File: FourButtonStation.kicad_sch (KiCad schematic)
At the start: 41 parts, among them J1 c8-inlet, J2 Conn_WallSocket, J3 I2C, J4 AVOX Adapter, J5 Conn_WallSocket, J6 USB_B_Micro, J7 Conn_WallSocket, J8 Conn_WallSocket, J9 I2C, K1 G5Q-1, K2 G5Q-1, K4 FINDER-36.11, K5 G5Q-1, Q1 MMBT3904, Q2 MMBT3904, Q3 MMBT3904, Q4 MMBT3904, Q5 MMBT3904, Q6 MMBT3904, SW3 RST, SW4 Boot, U1 CH340C, U2 radio-receiver, U3 ESP-07

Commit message: Schematic and routing
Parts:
- removed C1: TODO: 20u as SMD Package?, Capacitor_THT:CP_Radial_D5.0mm_P2.50mm, symbol Device:C_Polarized_Small
- removed D1: TODO: SMD Diodes Package, Diode_THT:D_DO-15_P2.54mm_Vertical_KathodeUp, symbol Device:D_Small
- removed D2, D3, D4: D_Small, Diode_THT:D_DO-15_P2.54mm_Vertical_KathodeUp, symbol Device:D_Small
- removed J2: Conn_WallSocket, TerminalBlock_Phoenix:TerminalBlock_Phoenix_MKDS-1,5-2_1x02_P5.00mm_Horizontal, symbol Connector:Conn_WallSocket
- removed J9: I2C, jlc_footprints:CONN-SMD_BM04B-SRSS-TB, symbol BM04B-SRSS-TB(LF)(SN):BM04B-SRSS-TB(LF)(SN)
- removed K1, K2, K5: G5Q-1, omron-g5sb-14:RELAY_G5SB-14_OMR, symbol Relay:G5Q-1
- removed K4: FINDER-36.11, omron-g5sb-14:RELAY_G5SB-14_OMR, symbol Relay:FINDER-36.11
- removed Q2, Q4, Q5, Q6: MMBT3904, jlc_footprints:SOT-23-3_L2.9-W1.3-P1.90-LS2.4-BR, symbol Transistor_BJT:MMBT3904
- removed R1: 33k, Resistor_SMD:R_0603_1608Metric_Pad0.98x0.95mm_HandSolder, symbol Device:R
- removed R4, R5, R6: TODO: 33k needs to be JLC Package, Resistor_SMD:R_0603_1608Metric_Pad0.98x0.95mm_HandSolder, symbol Device:R
- removed SW3: RST, jlc_footprints:SW-SMD_4P-L5.1-W5.1-P3.70-LS6.5-TL-2, symbol Switch:SW_Push
- removed SW4: Boot, jlc_footprints:SW-SMD_4P-L5.1-W5.1-P3.70-LS6.5-TL-2, symbol Switch:SW_Push
- added J10: AC IN, TerminalBlock_Phoenix:TerminalBlock_Phoenix_MKDS-1,5-2_1x02_P5.00mm_Horizontal, symbol Connector:Screw_Terminal_01x02
- added J2: External 3V, Connector_PinHeader_2.54mm:PinHeader_1x02_P2.54mm_Vertical, symbol Connector_Generic:Conn_01x02
- added J9: Conn_WallSocket, TerminalBlock_Phoenix:TerminalBlock_Phoenix_MKDS-1,5-2_1x02_P5.00mm_Horizontal, symbol Connector:Conn_WallSocket
- added K1, K2, K3, K4: G5LE-1, Relay_THT:Relay_SPDT_Omron-G5LE-1, symbol Relay:G5LE-1
- added LED1, LED2, LED3, LED4: KT-0603R, jlc_footprints:LED0603-RD, symbol jlc_symbols:KT-0603R
- added R1, R10, R6, R8: 33k, jlc_footprints:R0603, symbol jlc_symbols:0603WAF3302T5E
- added R4, R5, R7, R9: 1k, jlc_footprints:R0603, symbol jlc_symbols:0603WAF3302T5E
- added SW1: POWER, as12ap:as12ap, symbol Switch:SW_SPDT
- added SW2: RST, jlc_footprints:SW-SMD_4P-L5.1-W5.1-P3.70-LS6.5-TL-2, symbol TS-1187A-B-A-B:TS-1187A-B-A-B
- added SW5: Mode, jlc_footprints:SW-SMD_4P-L5.1-W5.1-P3.70-LS6.5-TL-2, symbol TS-1187A-B-A-B:TS-1187A-B-A-B
- added U10, U4, U6, U8: SM4007PL, jlc_footprints:SOD-123F_L2.8-W1.8-LS3.7-RD, symbol jlc_symbols:SM4007PL
- added U11, U5, U7, U9: D882_C9634, jlc_footprints:SOT-89-3_L4.5-W2.5-P1.50-LS4.2-BR, symbol jlc_symbols:D882_C9634
- J1: value c8-inlet -> AC IN; now left out of the parts list
- J3: value I2C -> TTL
- J4: value AVOX Adapter -> TODO: AVOX Adapter might need voltage divider
- J6: footprint Connector_USB:USB_Micro-B_Molex-105017-0001 -> jlc_footprints:MICRO-USB-SMD_1050171001
- R2, R3: footprint jlc_footprints:C0402 -> jlc_footprints:R0402
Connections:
- net +3V3: now also J3.4 (Pin_4), J4.3 (Pin_3), K1.5, K2.5, K3.5, K4.5, LED1.2 (A), LED2.2 (A), LED3.2 (A), LED4.2 (A), SW1.2 (B), U10.1 (C), U4.1 (C), U6.1 (C), U8.1 (C); no longer J3.2 (Pin_2), J4.1 (Pin_1), PS1.4 (+Vo)
- net AC1: now also K1.3
- net AC2: now also J7.1 (AC_P), K2.3
- net AC3: now also J8.1 (AC_P), K3.3; no longer J7.1 (AC_P)
- net AC4: now also J9.1 (AC_P), K4.3; no longer J8.1 (AC_P)
- net ADC: now also J4.2 (Pin_2); no longer J4.3 (Pin_3)
- net GND: now also J4.1 (Pin_1), J2.1 (Pin_1), SW2.3 (C), SW5.3 (C), U11.3 (E), U5.3 (E), U7.3 (E), U9.3 (E); no longer J4.2 (Pin_2)
- net GPIO0: now also U3.12 (GPIO0), SW5.1 (A)
- net Nullleiter: now also J10.1 (Pin_1), J9.2 (AC_N)
- net Phase: now also J10.2 (Pin_2), K1.1, K2.1, K3.1, K4.1
- net RESET: now also U3.1 (~{RST}), SW2.1 (A)
- net RX: now also J3.3 (Pin_3), U3.15 (GPIO3/RXD); no longer U3.16 (GPIO1/TXD)
- net RadioA: now also U3.13 (GPIO4)
- net RadioB: now also U3.11 (GPIO2)
- net RadioC: now also U3.10 (GPIO15); no longer U3.13 (GPIO4)
- net RadioD: now also U3.7 (GPIO13); no longer U3.11 (GPIO2)
- net Relay1: now also R1.1
- net Relay2: now also R6.1
- net Relay3: now also R8.1
- net Relay4: now also R10.1
- net TX: now also J3.2 (Pin_2), U3.16 (GPIO1/TXD); no longer U3.15 (GPIO3/RXD)
- removed net SCL: J3.4 (Pin_4), U3.10 (GPIO15)
- removed net SDA: J3.3 (Pin_3), U3.7 (GPIO13)
- new net: R1.2, U5.1 (B)
- new net: K4.2, R9.1, U10.2 (A), U11.2 (C)
- new net: LED4.1 (K), R9.2
- new net: LED2.1 (K), R5.2
- new net: R10.2, U11.1 (B)
- new net: LED3.1 (K), R7.2
- new net: K1.2, R4.1, U4.2 (A), U5.2 (C)
- new net: R6.2, U7.1 (B)
- new net: K2.2, R5.1, U6.2 (A), U7.2 (C)
- new net: K3.2, R7.1, U8.2 (A), U9.2 (C)
- new net: LED1.1 (K), R4.2
- new net: PS1.4 (+Vo), SW1.1 (A)
- new net: R8.2, U9.1 (B)
- new net POWX: J2.2 (Pin_2), SW1.3 (C)
- no-connect marks 12 -> 16
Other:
- note added: "Relay: G5LE14 3V Adafruit uses it: https://www.digikey.ch/de/products/detail/adafruit-industries-llc/3191/6193590 Footprint JLC C688864 (songle version)"
- note added: "TODO: - Exclude all from BOM what I will place my self - Add a warning sign - Add capacitors for 3v3"
- note removed: "TODO: - Add antenna to button module"
- moved on the sheet: J5

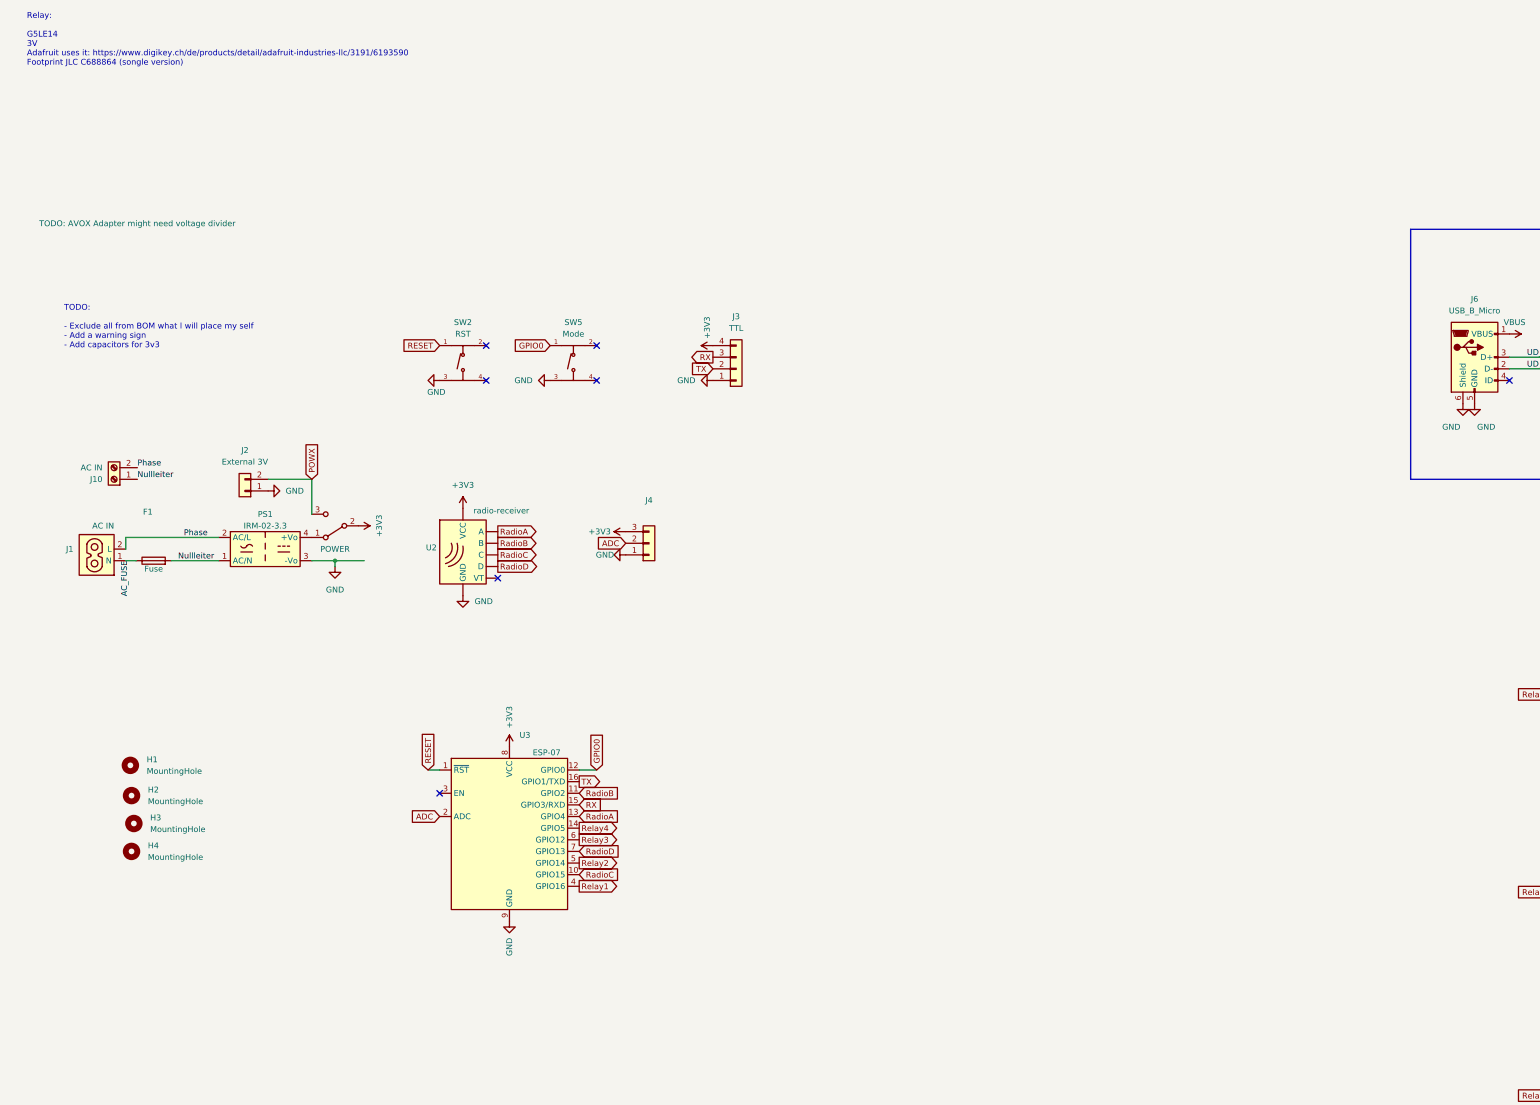
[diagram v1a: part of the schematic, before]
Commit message: Prepare for production
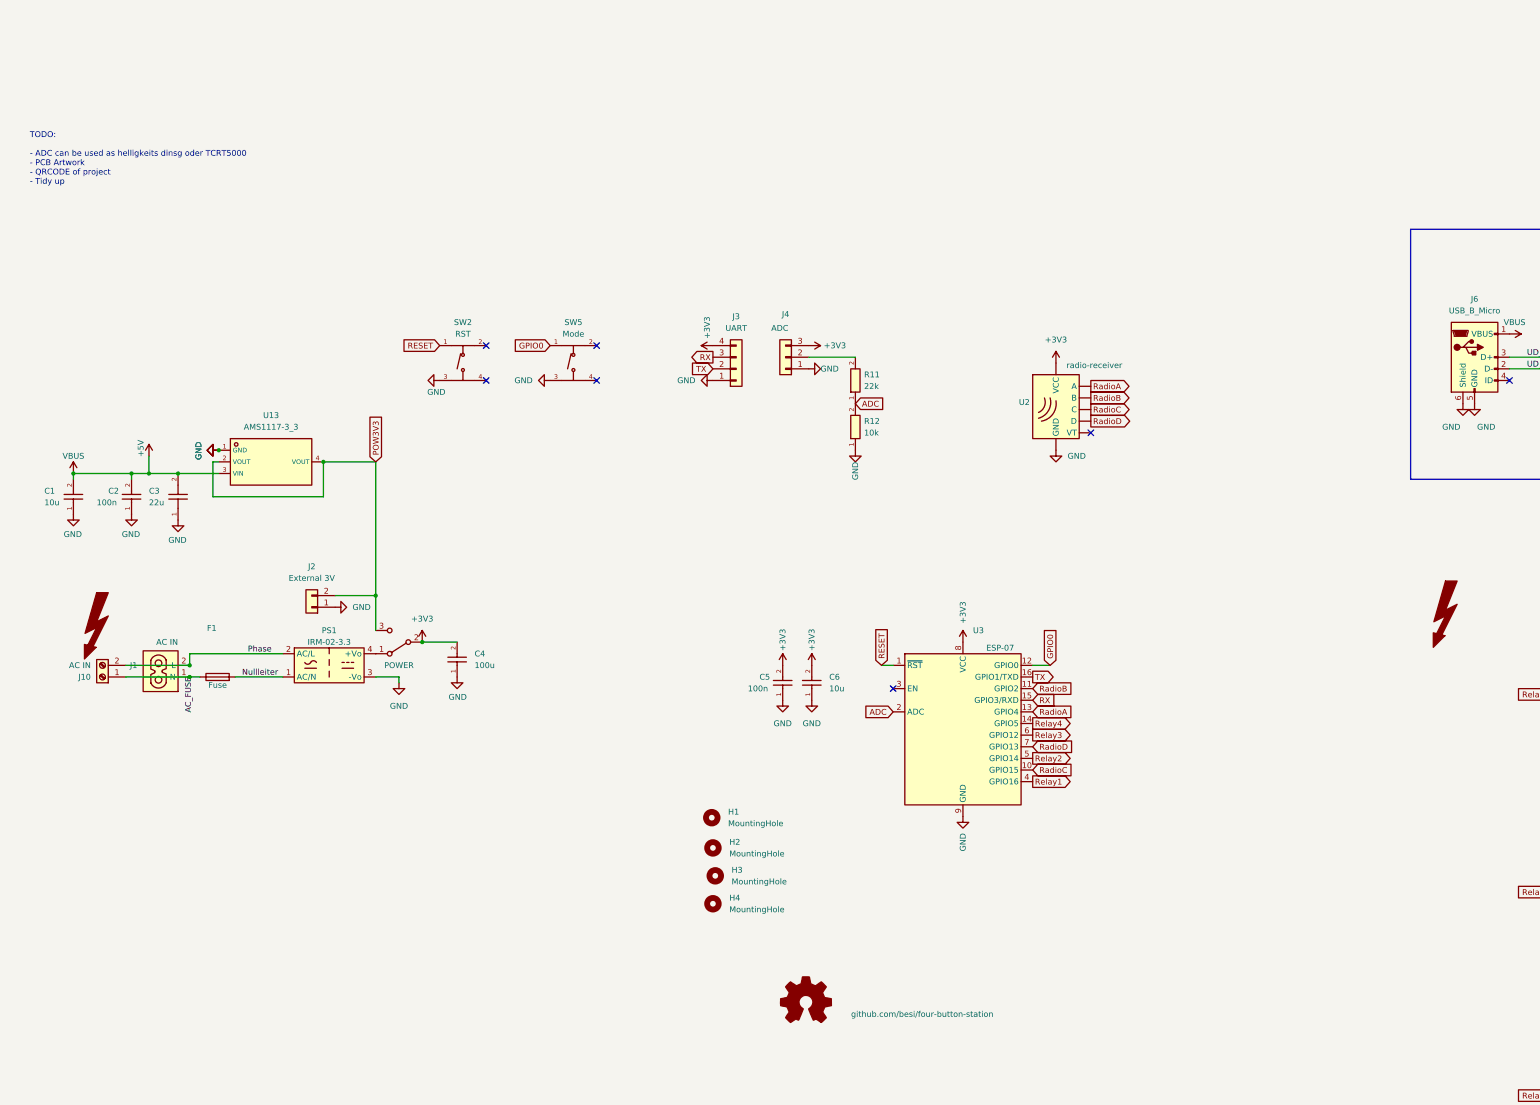
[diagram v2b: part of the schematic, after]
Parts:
- added C1, C6: 10u, jlc_footprints:C0402, symbol CL05A106MQ5NUNC:CL05A106MQ5NUNC
- added C2, C5: 100n, jlc_footprints:C0402, symbol CL05B104KO5NNNC:CL05B104KO5NNNC
- added C3: 22u, jlc_footprints:C0603, symbol CL10A226MQ8NRNC:CL10A226MQ8NRNC
- added C4: 100u, jlc_footprints:C1206, symbol CL31A107MQHNNNE:CL31A107MQHNNNE
- added R11: 22k, jlc_footprints:R0603, symbol jlc_symbols:0603WAF2202T5E
- added R12: 10k, jlc_footprints:R0603, symbol jlc_symbols:0603WAF1002T5E
- added SYM1: SYM_Flash_XLarge, Symbol:Symbol_HighVoltage_Type2_CopperTop_VerySmall, symbol Graphic:SYM_Flash_XLarge
- added Sym2: github.com/besi/four-button-station, Symbol:OSHW-Symbol_6.7x6mm_SilkScreen, symbol Graphic:Logo_Open_Hardware_Small
- added Sym3: SYM_Flash_XLarge, Symbol:EasterEgg_EWG1308-2013_ClassA, symbol Graphic:SYM_Flash_XLarge
- added U13: AMS1117-3_3, jlc_footprints:SOT-223-3_L6.5-W3.4-P2.30-LS7.0-BR, symbol jlc_symbols:AMS1117-3_3
- F1, H1, H2, H3, H4, J2, J5, J7, J8, J9, K1, K2, K3, K4, PS1, SW1, U2: now left out of the parts list
- J3: value TTL -> UART; now left out of the parts list
- J4: value TODO: AVOX Adapter might need voltage divider -> ADC; now left out of the parts list
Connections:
- net +3V3: now also C4.2, C5.2, C6.2
- net AC_FUSE: now also J10.1 (Pin_1)
- net ADC: now also R11.1, R12.2; no longer J4.2 (Pin_2)
- net GND: now also C1.1, C2.1, C3.1, C4.1, C5.1, C6.1, R12.1, U13.1 (GND)
- net Nullleiter: no longer J10.1 (Pin_1)
- net POWX renamed POW3V3
- net POW3V3: now also U13.2 (VOUT), U13.4 (VOUT)
- net VBUS renamed +5V
- net +5V: now also C1.2, C2.2, C3.2, U13.3 (VIN)
- new net: J4.2 (Pin_2), R11.2
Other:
- note added: "TODO: - ADC can be used as helligkeits dinsg oder TCRT5000 - PCB Artwork - QRCODE of project - Tidy up"
- note removed: "Relay: G5LE14 3V Adafruit uses it: https://www.digikey.ch/de/products/detail/adafruit-industries-llc/3191/6193590 Footprint JLC C688864 (songle version)"
- note removed: "TODO: - Exclude all from BOM what I will place my self - Add a warning sign - Add capacitors for 3v3"
- moved on the sheet: F1, H1, H2, H3, H4, J1, J10, J2, J4, PS1, U2, U3
